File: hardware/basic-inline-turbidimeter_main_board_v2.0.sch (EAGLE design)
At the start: 24 parts, among them IC1 MEGA8-AI

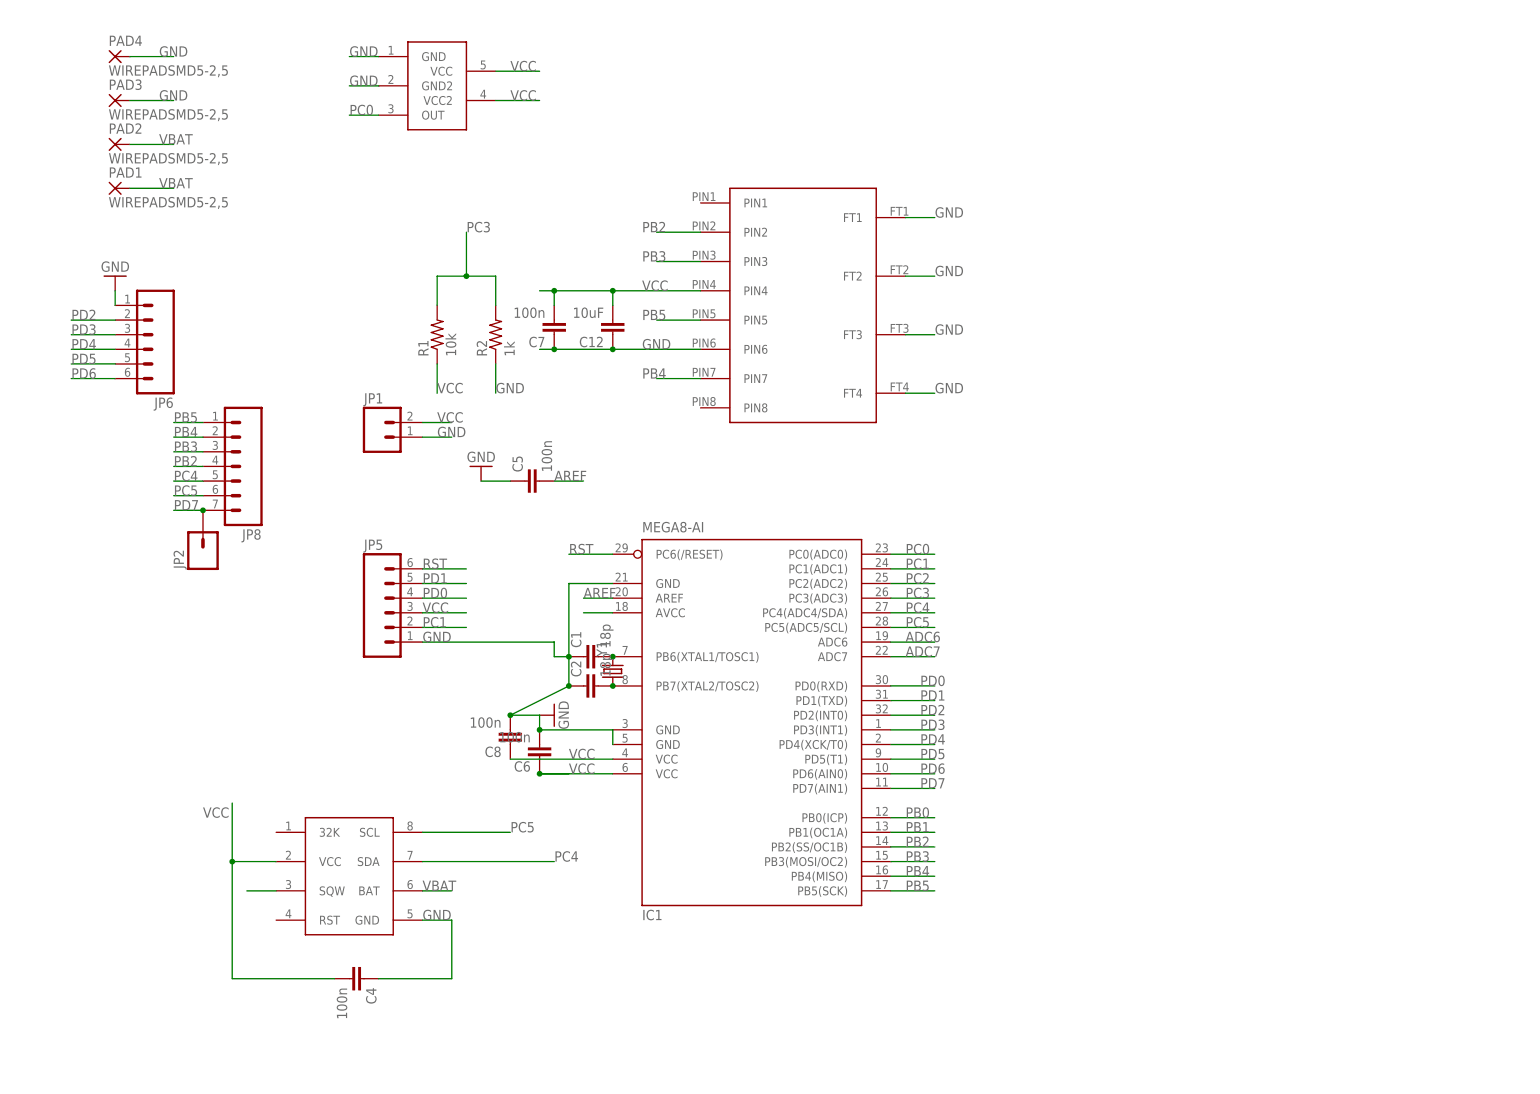
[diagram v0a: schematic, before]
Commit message: minor updates
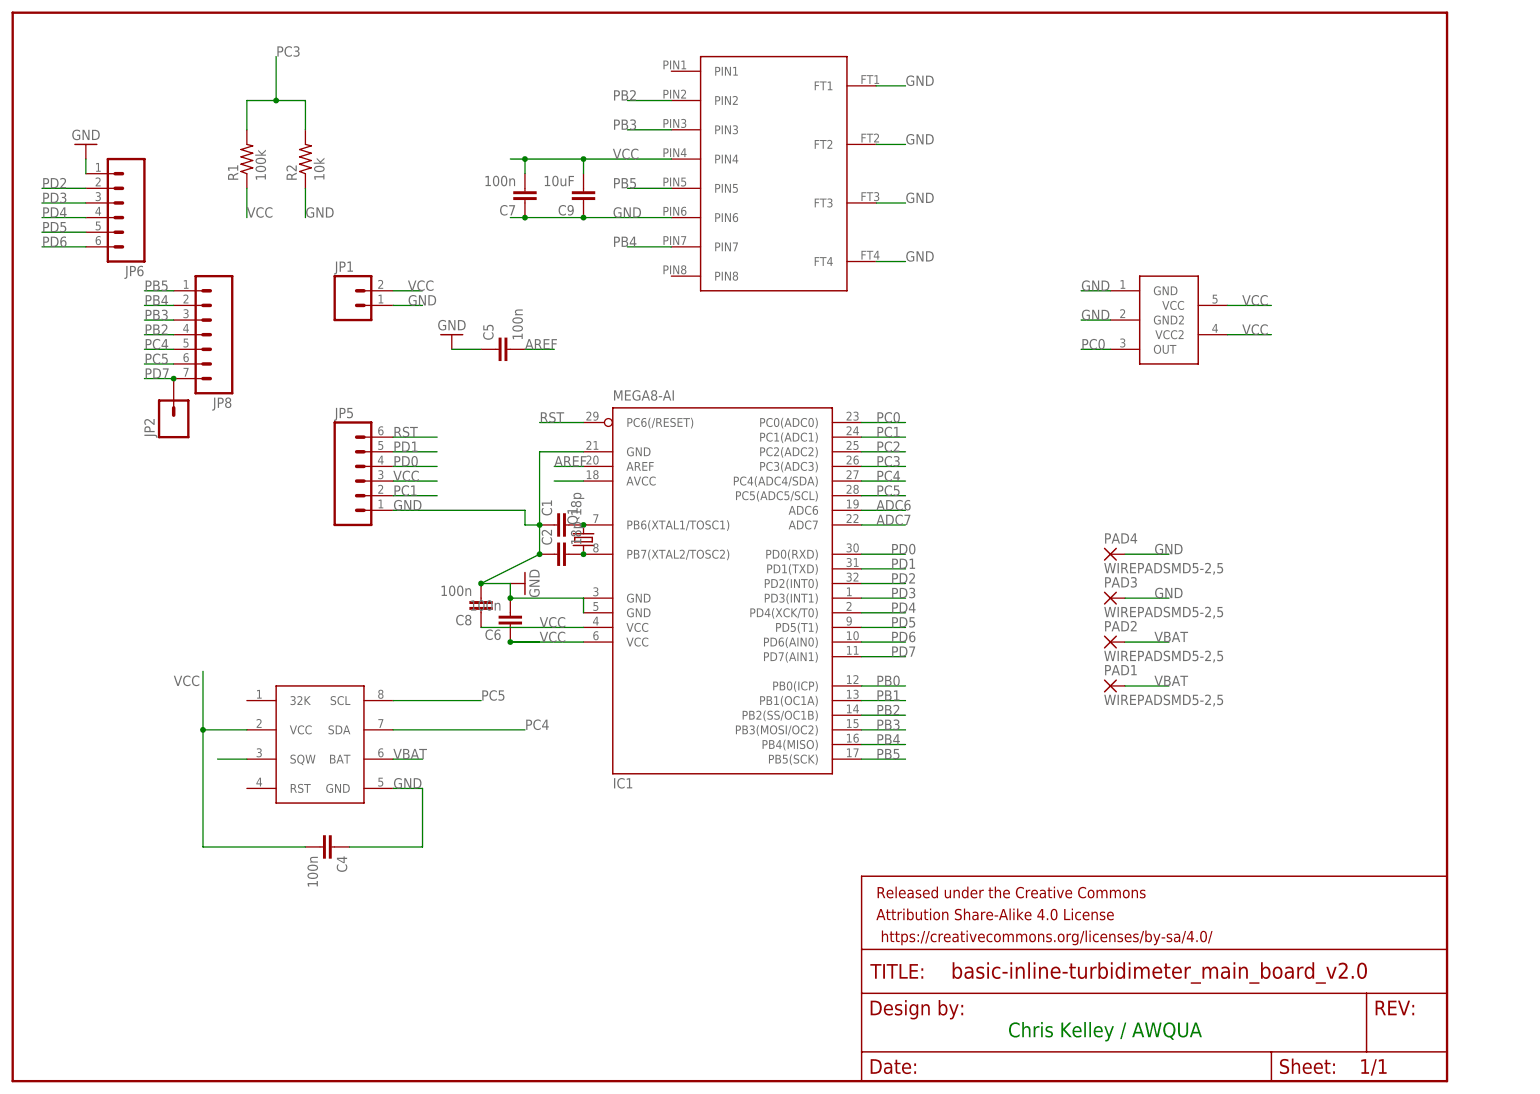
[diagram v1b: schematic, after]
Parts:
- removed C12: 10uF, SparkFun:CAP0603-CAP
- removed U$4: LMT86, open_source_turbidimeter:LMT86
- removed Y1: (no value), SparkFun:CRYSTAL5X3
- added C9: 10uF, SparkFun:CAP0603-CAP
- added FRAME1: FRAME-LETTER, SparkFun-Aesthetics:FRAME-LETTER
- added Q1: (no value), SparkFun:CRYSTAL5X3
- added T1: LMT86, open_source_turbidimeter:LMT86
- R1: value 10k -> 100k
- R2: value 1k -> 10k
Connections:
- net GND: now also C9.1, T1.GND, T1.GND2; no longer C12.1, U$4.GND, U$4.GND2
- net PC0: now also T1.OUT; no longer U$4.OUT
- net Q1: now also Q1.1; no longer Y1.1
- net Q2: now also Q1.2; no longer Y1.2
- net VCC: now also C9.2, T1.VCC, T1.VCC2; no longer C12.2, U$4.VCC, U$4.VCC2
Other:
- note added: "Chris Kelley / AWQUA"
- moved on the sheet: C1, C2, C4, C5, C6, C7, C8, IC1, JP1, JP2, JP5, JP6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
